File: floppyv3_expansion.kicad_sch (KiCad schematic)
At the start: 9 parts, among them J101 Conn_01x12_Socket, J102 Conn_01x12_Socket, J103 FTSH-107-01-L-DV-K-TR, J104 Conn_01x03_Socket, SW101 SW_Push

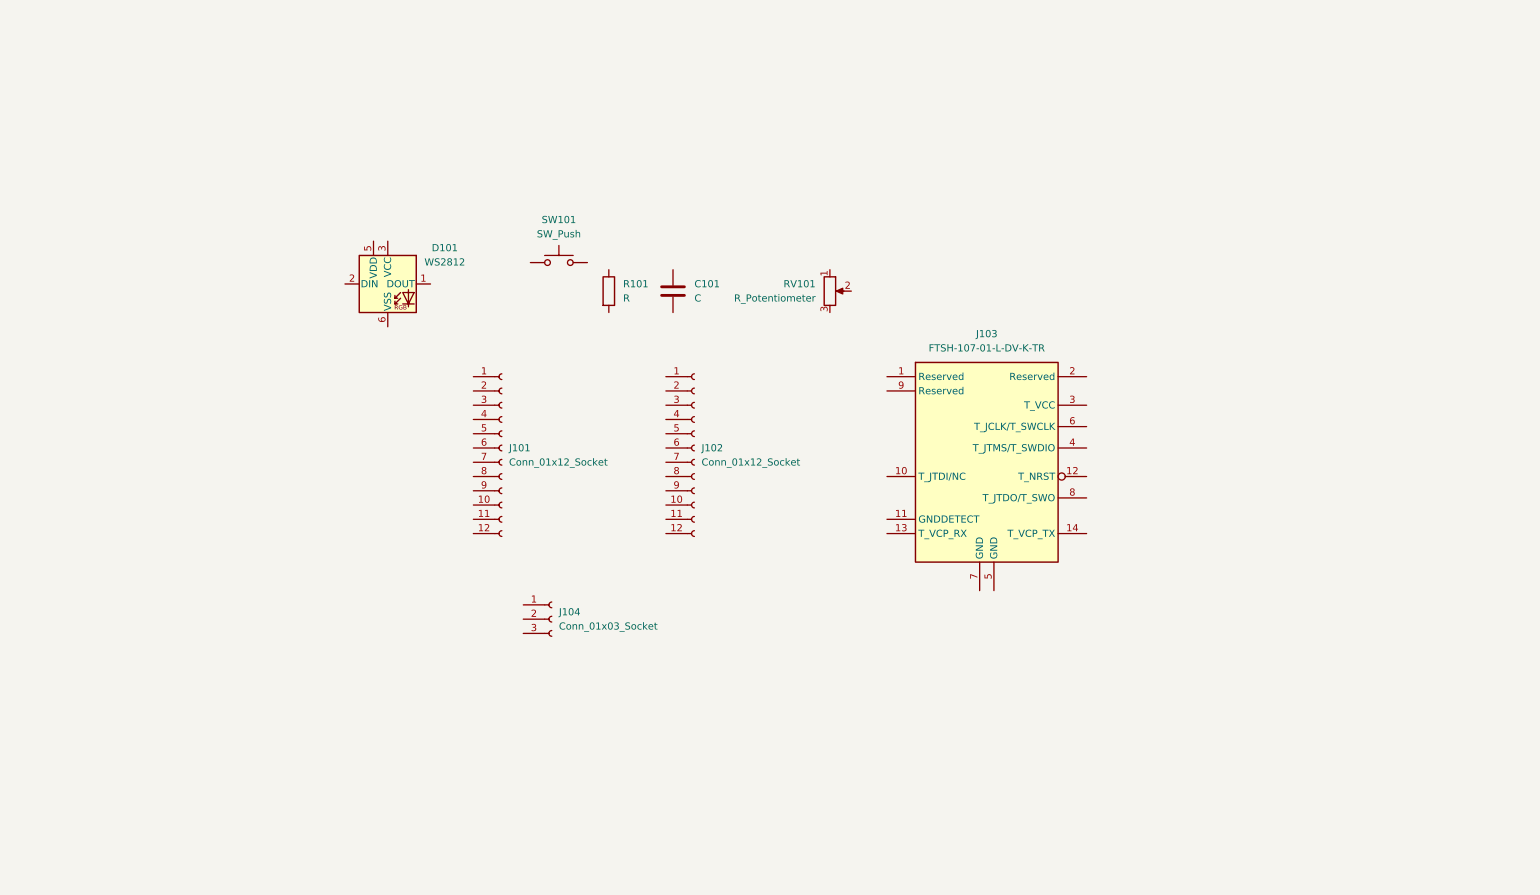
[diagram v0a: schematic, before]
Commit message: Almost finished v0.1
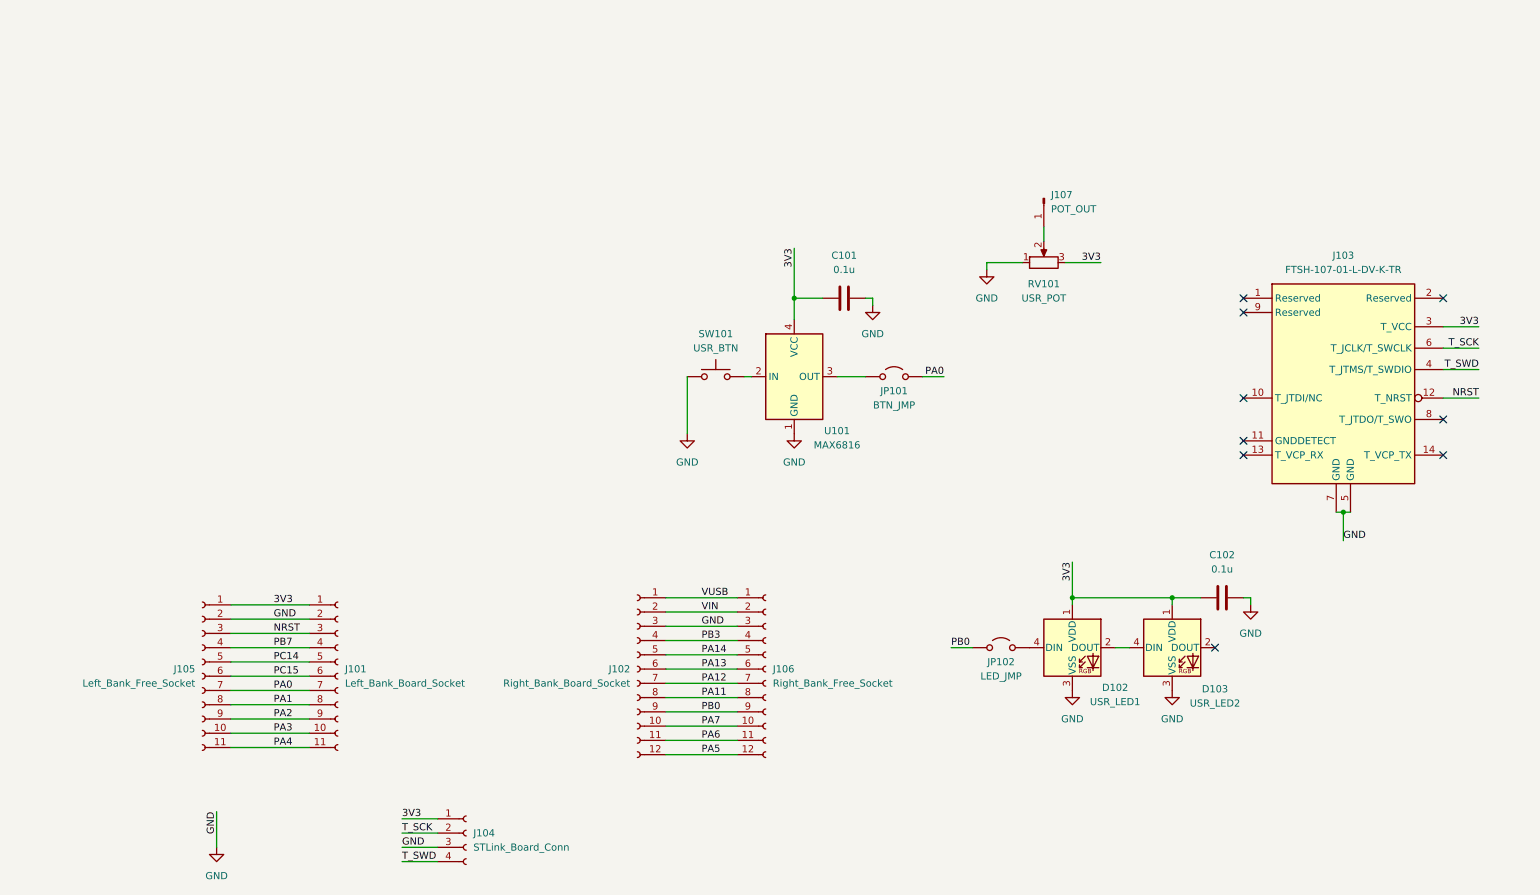
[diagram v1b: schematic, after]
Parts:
- removed D101: WS2812, LED_SMD:LED_WS2812_PLCC6_5.0x5.0mm_P1.6mm, symbol LED:WS2812
- removed R101: R, symbol Device:R
- added C102: 0.1u, Capacitor_SMD:C_0805_2012Metric, symbol Device:C
- added D102: USR_LED1, LED_SMD:LED_WS2812B_PLCC4_5.0x5.0mm_P3.2mm, symbol LED:WS2812B
- added D103: USR_LED2, LED_SMD:LED_WS2812B_PLCC4_5.0x5.0mm_P3.2mm, symbol LED:WS2812B
- added J105: Left_Bank_Free_Socket, Connector_PinSocket_2.54mm:PinSocket_1x12_P2.54mm_Vertical, symbol Connector:Conn_01x11_Socket
- added J106: Right_Bank_Free_Socket, Connector_PinSocket_2.54mm:PinSocket_1x11_P2.54mm_Vertical, symbol Connector:Conn_01x12_Socket
- added J107: POT_OUT, Connector_PinHeader_2.54mm:PinHeader_1x01_P2.54mm_Horizontal, symbol Connector:Conn_01x01_Pin
- added JP101: BTN_JMP, Connector_PinHeader_2.54mm:PinHeader_1x02_P2.54mm_Vertical, symbol Jumper:Jumper_2_Open
- added JP102: LED_JMP, Connector_PinHeader_2.54mm:PinHeader_1x02_P2.54mm_Vertical, symbol Jumper:Jumper_2_Open
- added U101: MAX6816, Package_TO_SOT_SMD:SOT-143, symbol Interface:MAX6816
- C101: value C -> 0.1u; footprint (none) -> Capacitor_SMD:C_0805_2012Metric
- J101: value Conn_01x12_Socket -> Left_Bank_Board_Socket; footprint (none) -> Connector_PinSocket_2.54mm:PinSocket_1x12_P2.54mm_Vertical; symbol Connector:Conn_01x12_Socket -> Connector:Conn_01x11_Socket
- J102: value Conn_01x12_Socket -> Right_Bank_Board_Socket; footprint (none) -> Connector_PinSocket_2.54mm:PinSocket_1x11_P2.54mm_Vertical
- J103: footprint FTSH10701LDVKTR -> (none)
- J104: value Conn_01x03_Socket -> STLink_Board_Conn; footprint (none) -> Connector_PinSocket_2.54mm:PinSocket_1x04_P2.54mm_Vertical; symbol Connector:Conn_01x03_Socket -> Connector:Conn_01x04_Socket
- RV101: value R_Potentiometer -> USR_POT; footprint (none) -> Potentiometer_THT:Potentiometer_Alps_RK09K_Single_Vertical
- SW101: value SW_Push -> USR_BTN
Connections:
- net 3V3: now reaches J101.1 (Pin_1)
- net 3V3: now also C101.1, J103.3 (T_VCC), J104.1 (Pin_1), RV101.3, C102.1, D102.1 (VDD), D103.1 (VDD), J105.1 (Pin_1), U101.4 (VCC)
- net PA3: now reaches J101.10 (Pin_10)
- net PA3: now also J105.10 (Pin_10)
- net PA4: now reaches J101.11 (Pin_11)
- net PA4: now also J105.11 (Pin_11)
- net GND: now reaches J101.2 (Pin_2)
- net GND: now also C101.2, J102.3 (Pin_3), J103.5 (GND), J103.7 (GND), J104.3 (Pin_3), RV101.1, SW101.1, C102.2, D102.3 (VSS), D103.3 (VSS), J105.2 (Pin_2), J106.3 (Pin_3), U101.1 (GND)
- net NRST: now reaches J101.3 (Pin_3)
- net NRST: now also J103.12 (T_NRST), J105.3 (Pin_3)
- net PB7: now reaches J101.4 (Pin_4)
- net PB7: now also J105.4 (Pin_4)
- net PC14: now reaches J101.5 (Pin_5)
- net PC14: now also J105.5 (Pin_5)
- net PC15: now reaches J101.6 (Pin_6)
- net PC15: now also J105.6 (Pin_6)
- net PA0: now reaches J101.7 (Pin_7)
- net PA0: now also J105.7 (Pin_7), JP101.2 (B)
- net PA1: now reaches J101.8 (Pin_8)
- net PA1: now also J105.8 (Pin_8)
- net PA2: now reaches J101.9 (Pin_9)
- net PA2: now also J105.9 (Pin_9)
- net VUSB: now reaches J102.1 (Pin_1)
- net VUSB: now also J106.1 (Pin_1)
- net PA7: now reaches J102.10 (Pin_10)
- net PA7: now also J106.10 (Pin_10)
- net PA6: now reaches J102.11 (Pin_11)
- net PA6: now also J106.11 (Pin_11)
- net PA5: now reaches J102.12 (Pin_12)
- net PA5: now also J106.12 (Pin_12)
- net VIN: now reaches J102.2 (Pin_2)
- net VIN: now also J106.2 (Pin_2)
- net PB3: now reaches J102.4 (Pin_4)
- net PB3: now also J106.4 (Pin_4)
- net PA14: now reaches J102.5 (Pin_5)
- net PA14: now also J106.5 (Pin_5)
- net PA13: now reaches J102.6 (Pin_6)
- net PA13: now also J106.6 (Pin_6)
- net PA12: now reaches J102.7 (Pin_7)
- net PA12: now also J106.7 (Pin_7)
- net PA11: now reaches J102.8 (Pin_8)
- net PA11: now also J106.8 (Pin_8)
- net PB0: now reaches J102.9 (Pin_9)
- net PB0: now also J106.9 (Pin_9), JP102.1 (A)
- net T_SCK: now reaches J104.2 (Pin_2)
- net T_SCK: now also J103.6 (T_JCLK/T_SWCLK)
- net at RV101.2: now also J107.1 (Pin_1)
- net at SW101.2: now also U101.2 (IN)
- net T_SWD: now reaches J103.4 (T_JTMS/T_SWDIO)
- net T_SWD: now also J104.4 (Pin_4)
- new net: JP101.1 (A), U101.3 (OUT)
- new net: D102.2 (DOUT), D103.4 (DIN)
- new net: D102.4 (DIN), JP102.2 (B)
- no-connect marks 0 -> 9
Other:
- moved on the sheet: J102, J103, RV101, SW101

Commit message: Started layout
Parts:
- J101, J105: footprint Connector_PinSocket_2.54mm:PinSocket_1x12_P2.54mm_Vertical -> Connector_PinSocket_2.54mm:PinSocket_1x11_P2.54mm_Vertical
- J102, J106: footprint Connector_PinSocket_2.54mm:PinSocket_1x11_P2.54mm_Vertical -> Connector_PinSocket_2.54mm:PinSocket_1x12_P2.54mm_Vertical
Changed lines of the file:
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@@
 			"AAAAAAAAAAAAAAAAAAAAAAAAAAAAAAAAAAAAAAAAAAAAAAAAAAAAAAAAAAAAAAAAAAAAAAAAAAAA"
 			"AAAAAAAAAAAAAAAAAAAAAAAAAAAAAAAAAAAAAAAAAAAAAAAAAAAAAAAAAAAAAAAAAAAAAAAAAAAA"
-			"AAAAAAAA"
+			"AAAAAAAAAAAAAAAAAAAAAAAAAAAAAAAAAAAAAAAAAAAAAAAAAAAAAAAAAAAAAAAAAAAAAAAAAAAA"
+			"AAAAAAAAAAAAAAAAAAAAAAAAAAAAAAAAAAAAAAAAAAAAAAAAAAAAAAAAAAAAAAAAAAAAAAAAAAAA"
+			"AAAAAAAAAAAAAAAAAAAAAAAAAAAAAAAAAAAAAAAAAAAAAAAAAAAAAAAAAAAAAAAAAAAAAAAAAAAA"
+			"AAAAAAAAAAAAAAAAAAAAAAAAAAAAAAAAAAAAAAAAAAAAAAAAAAAAAAAAAAAAAAAAAAAAAAAAAAAA"
+			"AAAAAAAAAAAAAAAAAAAAAAAAAAAAAAAAAAAAAAAAAAAAAAAAAAAAAAAAAAAAAAAAAAAAAAAAAAAA"
+			"AAAAAAAAAAAAAAAAAAAAAAAAAAAAAAAAAAAAAAAAAAAAAAAAAAAAAAAAAAAAAAAAAAAAAAAAAAAA"
+			"AAAAAAAAAAAAAAAAAAAAAAAAAAAAAAAAAAAAAAAAAAAAAAAAAAAAAAAAAAAAAAAAAAAAAAAAAAAA"
+			"AAAAAAAAAAAAAAAAAAAAAAAAAAAAAAAAAAAAAAAAAAAAAAAAAAAAAAAAAAAAAAAAAAAAAAAAAAAA"
+			"AAAAAAAAAAAAAAAAAAAAAAAAAAAAAAAAAAAAAAAAAAAAAAAAAAAAAAAAAAAAAAAAAAAAAAAAAAAA"
+			"AAAAAAAAAAAAAAAAAAAAAAAAAAAAAAAAAAAAAAAAAAAAAAAAAAAAAAAAAAAAAAAAAAAAAAAAAAAA"
+			"AAAAAAAAAAAAAAAAAAAAAAAAAAAAAAAAAAAAAAAAAAAAAAAAAAAAAAAAAAAAAAAAAAAAAAAAAAAA"
+			"AAAAAAAAAAAAAAAAAAAAAAAAAAAAAAAAAAAAAAAAAAAAAAAAAAAAAAAAAAAAAAAAAAAAAAAAAAAA"
+			"AAAAAAAAAAAAAAAAAAAAAAAAAAAAAAAAAAAAAAAAAAAAAAAAAAAAAAAAAAAAAAAAAAAAAAAAAAAA"
+			"AAAAAAAAAAAAAAAAAAAAAAAAAAAAAAAAAAAAAAAAAAAAAAAAAAAAAAAAAAAAAAAAAAAAAAAAAAAA"
+			"AAAAAAAAAAAAAAAAAAAAAAAAAAAAAAAAAAAAAAAAAAAAAAAAAAAAAAAAAAAAAAAAAAAAAAAAAAAA"
+			"AAAAAAAAAAAAAAAAAAAAAAAAAAAAAAAAAAAAAAAAAAAAAAAAAAAAAAAAAAAAAAAAAAAAAAAAAAAA"
+			"AAAAAAAAAAAAAAAAAAAAAAAAAAAAAAAAAAAAAAAAAAAAAAAAAAAAAAAAAAAAAAAAAAAAAAAAAAAA"
+			"AAAAAAAAAAAAAAAAAAAAAAAAAAAAAAAAAAAAAAAAAAAAAAAAAAAAAAAAAAAAAAAAAAAAAAAAAAAA"
+			"AAAAAA=="
 		)
 	)
@@
 			)
 		)
-		(property "Footprint" "Connector_PinSocket_2.54mm:PinSocket_1x12_P2.54mm_Vertical"
+		(property "Footprint" "Connector_PinSocket_2.54mm:PinSocket_1x11_P2.54mm_Vertical"
 			(at 72.39 135.89 0)
 			(effects
@@
 			)
 		)
-		(property "Footprint" "Connector_PinSocket_2.54mm:PinSocket_1x12_P2.54mm_Vertical"
+		(property "Footprint" "Connector_PinSocket_2.54mm:PinSocket_1x11_P2.54mm_Vertical"
 			(at 48.26 135.89 0)
 			(effects
@@
 			)
 		)
-		(property "Footprint" "Connector_PinSocket_2.54mm:PinSocket_1x11_P2.54mm_Vertical"
+		(property "Footprint" "Connector_PinSocket_2.54mm:PinSocket_1x12_P2.54mm_Vertical"
 			(at 125.73 134.62 0)
 			(effects
@@
 			)
 		)
-		(property "Footprint" "Connector_PinSocket_2.54mm:PinSocket_1x11_P2.54mm_Vertical"
+		(property "Footprint" "Connector_PinSocket_2.54mm:PinSocket_1x12_P2.54mm_Vertical"
 			(at 148.59 134.62 0)
 			(effects

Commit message: Starting to layout components
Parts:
- J103: footprint (none) -> SAMTEC_FTSH-107-01-L-DV-K-TR:SAMTEC_FTSH-107-01-L-DV-K-TR; symbol SAMTEC-FTSH-107-01-L-DV-K-TR:FTSH-107-01-L-DV-K-TR -> SAMTEC_FTSH_107_01_L_DV_K_TR:FTSH-107-01-L-DV-K-TR
- J107: footprint Connector_PinHeader_2.54mm:PinHeader_1x01_P2.54mm_Horizontal -> Connector_PinHeader_2.54mm:PinHeader_1x01_P2.54mm_Vertical
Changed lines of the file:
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@@
+			"AAAAAAAAAAAAAAAAAAAAAAAAAAAAAAAAAAAAAAAAAAAAAAAAAAAAAAAAAAAAAAAAAAAAAAAAAAAA"
+			"AAAAAAAAAAAAAAAAAAAAAAAAAAAAAAAAAAAAAAAAAAAAAAAAAAAAAAAAAAAAAAAAAAAAAAAAAAAA"
+			"AAAAAAAAAAAAAAAAAAAAAAAAAAAAAAAAAAAAAAAAAAAAAAAAAAAAAAAAAAAAAAAAAAAAAAAAAAAA"
+			"AAAAAAAAAAAAAAAAAAAAAAAAAAAAAAAAAAAAAAAAAAAAAAAAAAAAAAAAAAAAAAAAAAAAAAAAAAAA"
+			"AAAAAAAAAAAAAAAAAAAAAAAAAAAAAAAAAAAAAAAAAAAAAAAAAAAAAAAAAAAAAAAAAAAAAAAAAAAA"
+			"AAAAAAAAAAAAAAAAAAAAAAAAAAAAAAAAAAAAAAAAAAAAAAAAAAAAAAAAAAAAAAAAAAAAAAAAAAAA"
+			"AAAAAAAAAAAAAAAAAAAAAAAAAAAAAAAAAAAAAAAAAAAAAAAAAAAAAAAAAAAAAAAAAAAAAAAAAAAA"
+			"AAAAAAAAAAAAAAAAAAAAAAAAAAAAAAAAAAAAAAAAAAAAAAAAAAAAAAAAAAAAAAAAAAAAAAAAAAAA"
+			"AAAAAAAAAAAAAAAAAAAAAAAAAAAAAAAAAAAAAAAAAAAAAAAAAAAAAAAAAAAAAAAAAAAAAAAAAAAA"
+			"AAAAAAAAAAAAAAAAAAAAAAAAAAAAAAAAAAAAAAAAAAAAAAAAAAAAAAAAAAAAAAAAAAAAAAAAAAAA"
+			"AAAAAAAAAAAAAAAAAAAAAAAAAAAAAAAAAAAAAAAAAAAAAAAAAAAAAAAAAAAAAAAAAAAAAAAAAAAA"
+			"AAAAAAAAAAAAAAAAAAAAAAAAAAAAAAAAAAAAAAAAAAAAAAAAAAAAAAAAAAAAAAAAAAAAAAAAAAAA"
+			"AAAAAAAAAAAAAAAAAAAAAAAAAAAAAAAAAAAAAAAAAAAAAAAAAAAAAAAAAAAAAAAAAAAAAAAAAAAA"
+			"AAAAAAAAAAAAAAAAAAAAAAAAAAAAAAAAAAAAAAAAAAAAAAAAAAAAAAAAAAAAAAAAAAAAAAAAAAAA"
+			"AAAAAAAAAAAAAAAAAAAAAAAAAAAAAAAAAAAAAAAAAAAAAAAAAAAAAAAAAAAAAAAAAAAAAAAAAAAA"
+			"AAAAAAAAAAAAAAAAAAAAAAAAAAAAAAAAAAAAAAAAAAAAAAAAAAAAAAAAAAAAAAAAAAAAAAAAAAAA"
+			"AAAAAAAAAAAAAAAAAAAAAAAAAAAAAAAAAAAAAAAAAAAAAAAAAAAAAAAAAAAAAAAAAAAAAAAAAAAA"
+			"AAAAAAAAAAAAAAAAAAAAAAAAAAAAAAAAAAAAAAAAAAAAAAAAAAAAAAAAAAAAAAAAAAAAAAAAAAAA"
 			"AAAAAAAAAAAAAAAAAAAAAAAAAAAAAAAAAAAAAAAAAAAAAAAAAAAAAAAAAAAAAAAAAAAAAAAAAAAA"
 			"AAAAAAAAAAAAAAAAAAAAAAAAAAAAAAAAAAAAAAAAAAAAAAAAAAAAAAAAAAAAAAAAAAAAAAAAAAAA"
@@
 			)
 		)
-		(property "Footprint" "Connector_PinHeader_2.54mm:PinHeader_1x01_P2.54mm_Horizontal"
+		(property "Footprint" "Connector_PinHeader_2.54mm:PinHeader_1x01_P2.54mm_Vertical"
 			(at 198.12 50.8 0)
 			(effects
@@
 	)
 	(symbol
-		(lib_id "SAMTEC-FTSH-107-01-L-DV-K-TR:FTSH-107-01-L-DV-K-TR")
+		(lib_id "SAMTEC_FTSH_107_01_L_DV_K_TR:FTSH-107-01-L-DV-K-TR")
 		(at 233.68 68.58 0)
 		(unit 1)
@@
 			)
 		)
-		(property "Footprint" ""
+		(property "Footprint" "SAMTEC_FTSH-107-01-L-DV-K-TR:SAMTEC_FTSH-107-01-L-DV-K-TR"
 			(at 252.73 163.5 0)
 			(effects

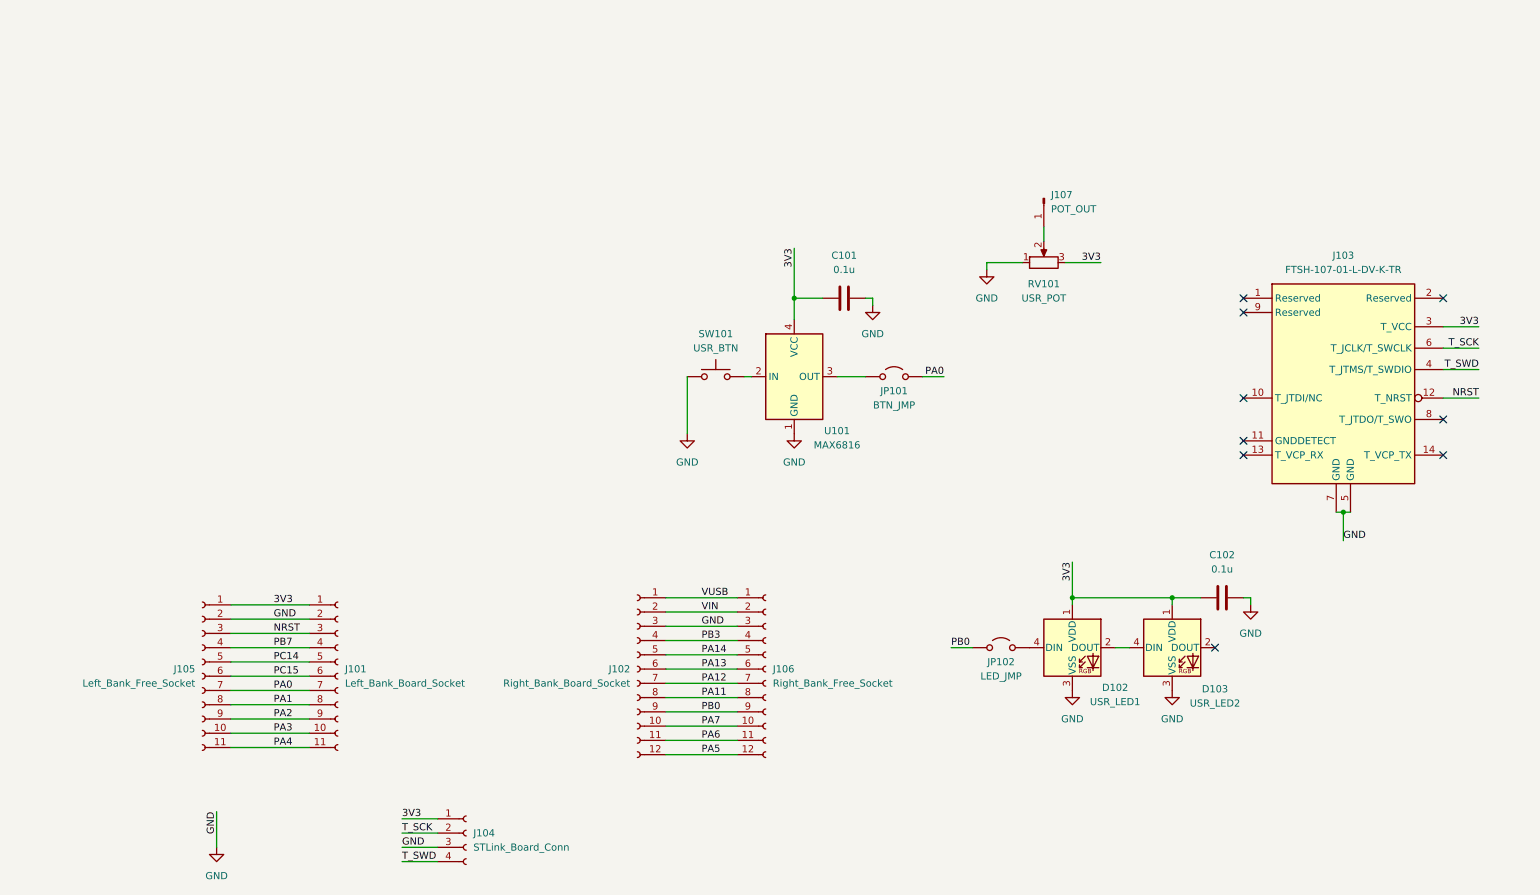
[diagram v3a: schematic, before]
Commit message: Further improvements to layout and schematic
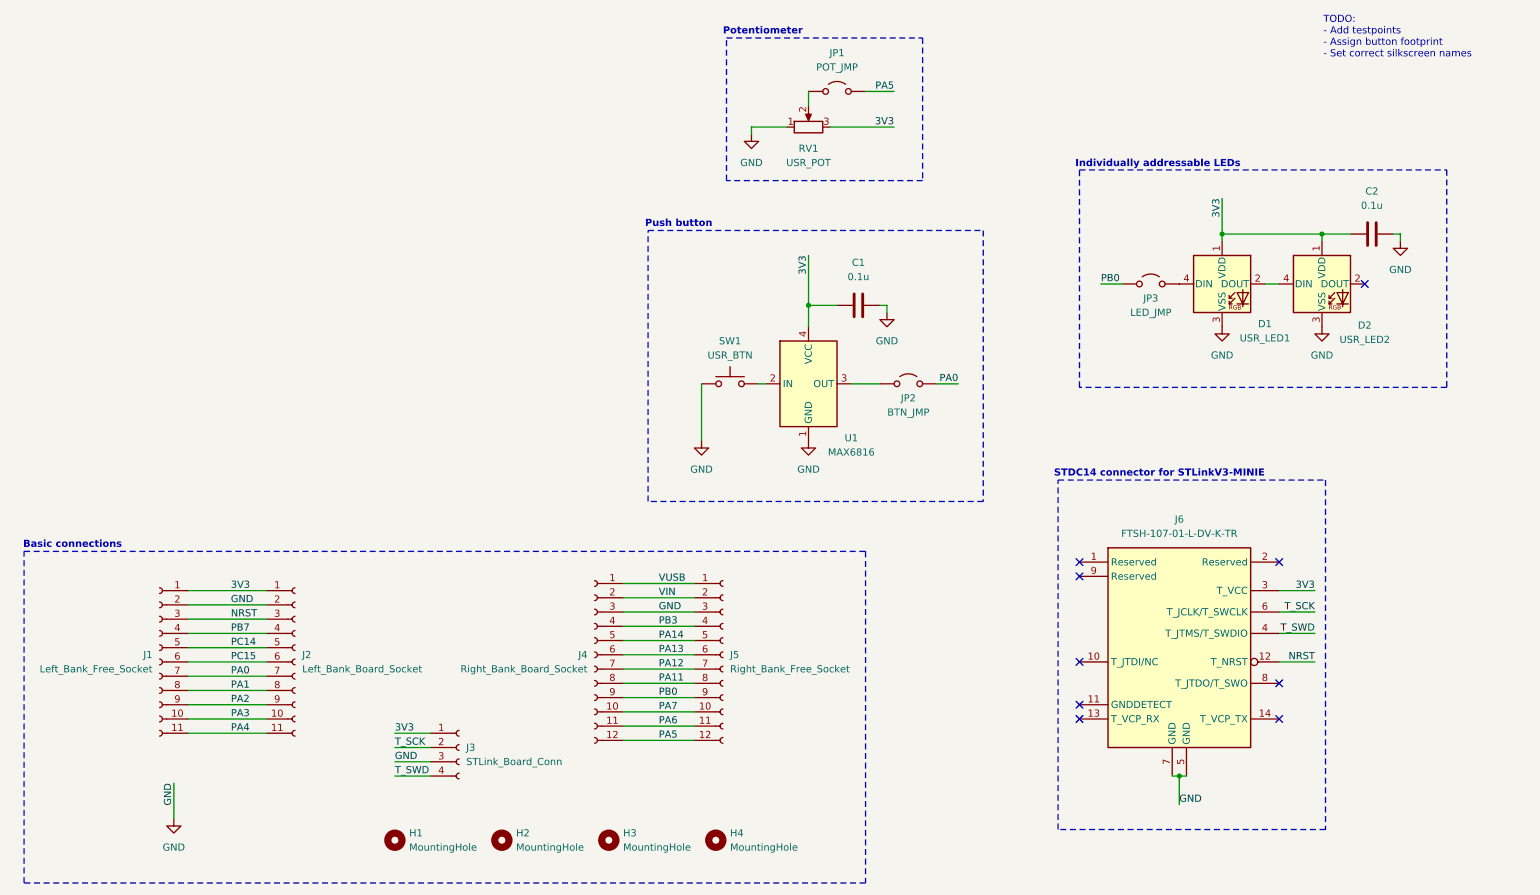
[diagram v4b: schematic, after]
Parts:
- removed J107: POT_OUT, Connector_PinHeader_2.54mm:PinHeader_1x01_P2.54mm_Vertical, symbol Connector:Conn_01x01_Pin
- added H1, H2, H3, H4: MountingHole, MountingHole:MountingHole_2.2mm_M2_Pad_Via, symbol Mechanical:MountingHole
- added JP1: POT_JMP, Connector_PinHeader_2.54mm:PinHeader_1x02_P2.54mm_Vertical, symbol Jumper:Jumper_2_Open
- SW1: renamed from SW101; footprint (none) -> Button_Switch_THT:SW_PUSH-12mm
- renumbered C101 to C1, C102 to C2, D102 to D1, D103 to D2, J105 to J1, J101 to J2, J104 to J3, J102 to J4, J106 to J5, J103 to J6, JP101 to JP2, JP102 to JP3, RV101 to RV1, U101 to U1
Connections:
- net PA5: now also JP1.2 (B)
- net at RV1.2: now also JP1.1 (A)
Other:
- note added: "Basic connections"
- note added: "Individually addressable LEDs"
- note added: "Potentiometer"
- note added: "Push button"
- note added: "STDC14 connector for STLinkV3-MINIE"
- note added: "TODO: - Add testpoints - Assign button footprint - Set correct silkscreen names"
- moved on the sheet: C1, C2, D1, D2, J1, J2, J3, J4, J5, J6, JP2, JP3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
